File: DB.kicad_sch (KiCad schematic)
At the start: 10 parts

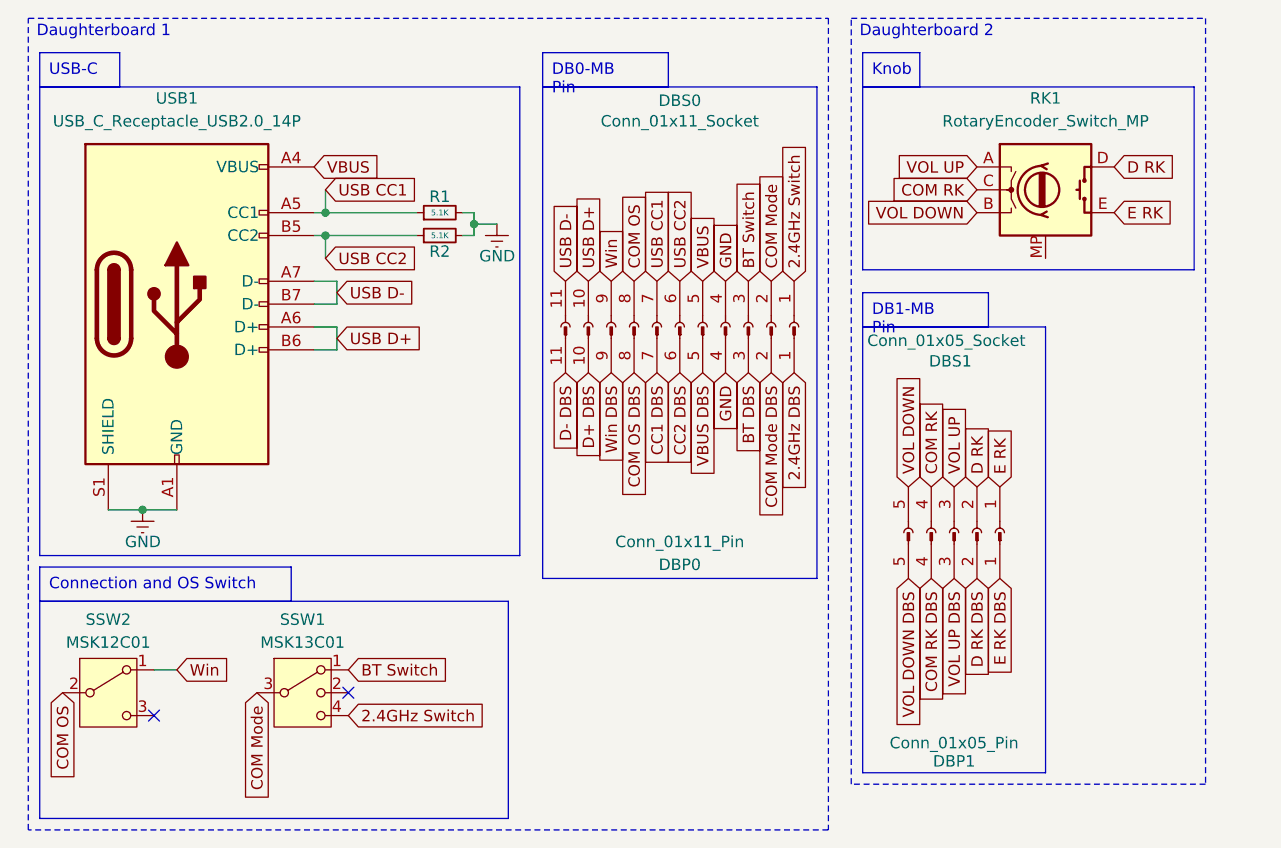
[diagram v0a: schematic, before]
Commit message: Sixth Commit
Almost done. Just need to make sure the field zone and each pin is connected properly
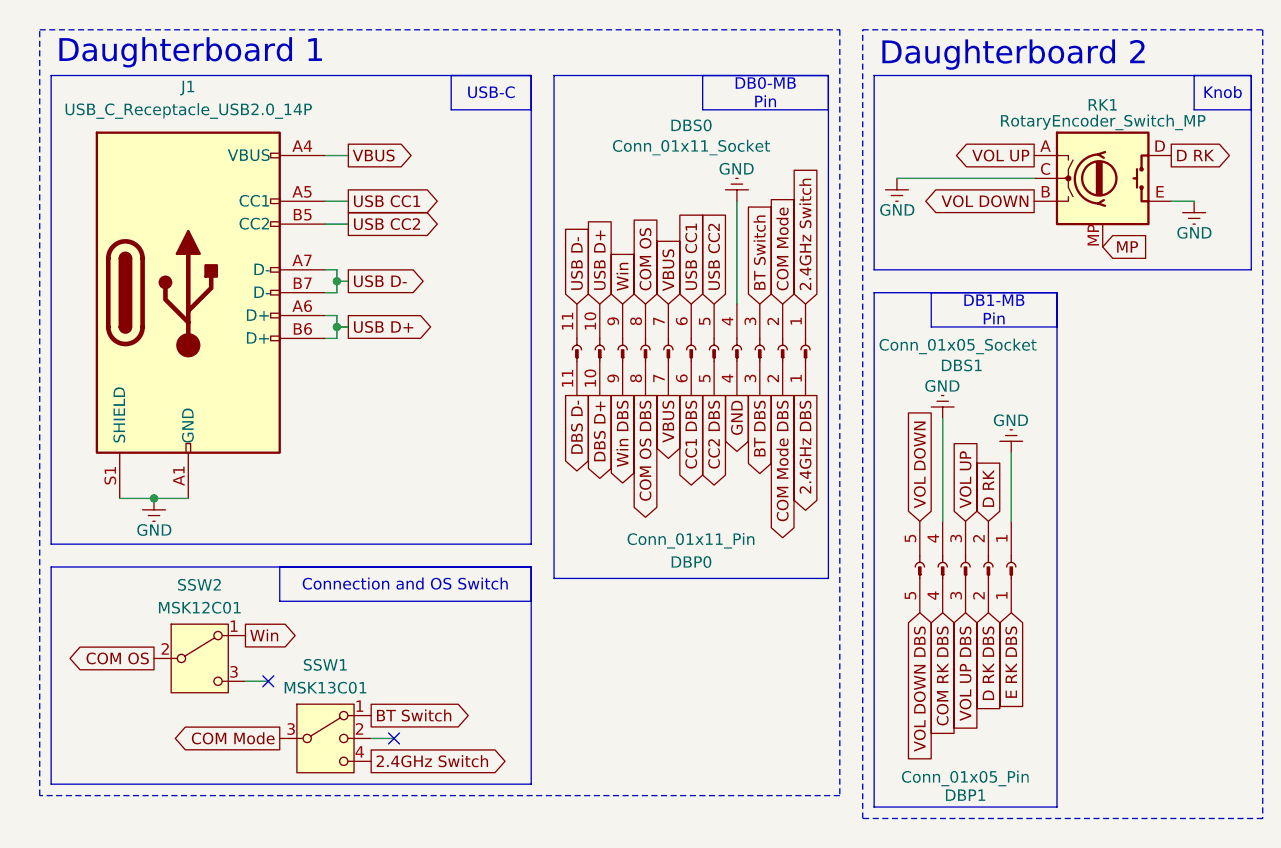
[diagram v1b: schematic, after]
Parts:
- removed R1, R2: 5.1K, ScottoKeebs_Components:Resistor_0402, symbol Device:R_Small
- J1: renamed from USB1; symbol Connector:USB_C_Receptacle_USB2.0_14P -> HE_Keyswitch:USB_C_Receptacle_USB2.0_14P
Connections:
- net COM RK is gone; now on net GND: DBS1.4 (Pin_4), RK1.C
- net E RK is gone; now on net GND: DBS1.1 (Pin_1), RK1.E (S2)
- net VBUS DBS is gone; now on net CC2 DBS: DBP0.5 (Pin_5)
- net CC1 DBS: now also DBP0.6 (Pin_6); no longer DBP0.7 (Pin_7)
- net CC2 DBS: no longer DBP0.6 (Pin_6)
- net USB CC1: now also DBS0.6 (Pin_6); no longer DBS0.7 (Pin_7)
- net USB CC2: now also DBS0.5 (Pin_5); no longer DBS0.6 (Pin_6)
- net VBUS: now also DBP0.7 (Pin_7), DBS0.7 (Pin_7); no longer DBS0.5 (Pin_5)
- net MP: now reaches RK1.MP
- net D+ DBS renamed DBS D+
- net D- DBS renamed DBS D-
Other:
- moved on the sheet: DBP0, DBP1, DBS0, DBS1, J1, RK1, SSW1, SSW2
